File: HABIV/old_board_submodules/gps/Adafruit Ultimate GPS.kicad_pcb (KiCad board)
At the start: 4 copper layers, 13 parts, among them U3 FGPMMOPA6H

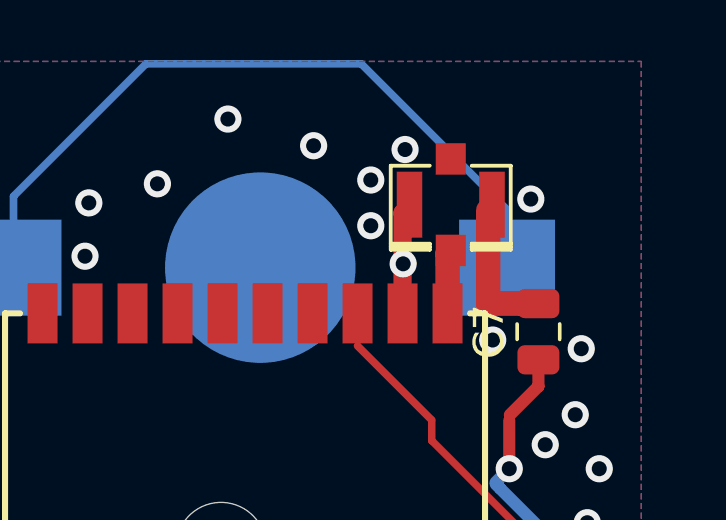
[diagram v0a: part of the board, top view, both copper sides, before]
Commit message: finish submodules and combine
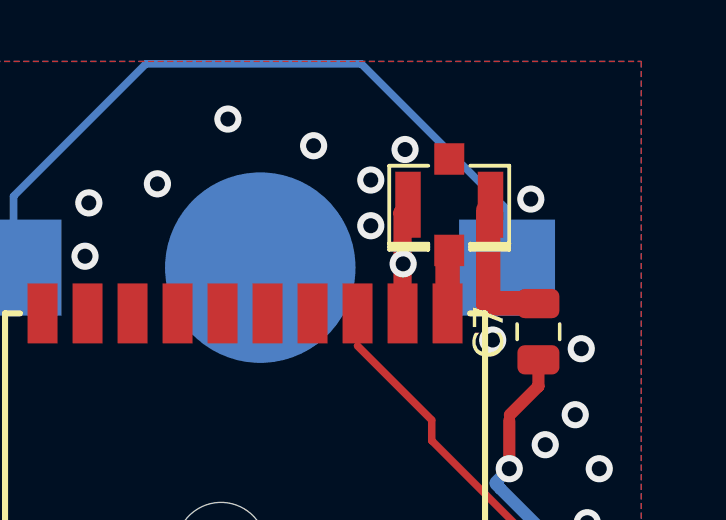
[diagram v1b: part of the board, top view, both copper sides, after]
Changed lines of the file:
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@@
   )
   (module "Adafruit Ultimate GPS:U.FL" (layer Top)
-    (at 154.85 93 270)
+    (at 154.8 93 270)
     (fp_text reference U$1 (at 0 0 270) (layer F.SilkS) hide
       (effects (font (size 1.27 1.27) (thickness 0.15)) (justify right top))
@@
   (segment (start 157.453199 105.546801) (end 157 106) (width 0.25) (layer Top) (net 3))
   (segment (start 154.2161 100.1776) (end 154.2161 100.864362) (width 0.25) (layer Top) (net 3))
-  (segment (start 153.2431 114.3586) (end 153.2431 112.6226) (width 0.4064) (layer Top) (net 9) (status 20))
   (segment (start 138.0771 99.0346) (end 137.9841 99.1276) (width 0.4064) (layer Top) (net 4) (status 30))
   (via (at 147.8 115.6) (size 0.9064) (drill 0.5) (layers Top Bottom) (net 4))
@@
   (segment (start 157.15 118.575) (end 155.85 119.875) (width 0.406) (layer Top) (net 8))
   (segment (start 159.3 118.575) (end 157.15 118.575) (width 0.406) (layer Top) (net 8))
+  (segment (start 153.2431 114.3586) (end 153.2431 112.6226) (width 0.4064) (layer Top) (net 9) (status 20))
   (segment (start 153.2431 117.7569) (end 153 118) (width 0.4064) (layer Top) (net 9))
   (segment (start 153.2431 112.6226) (end 153.2431 117.7569) (width 0.4064) (layer Top) (net 9))
